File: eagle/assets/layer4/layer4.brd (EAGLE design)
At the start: 102.9 x 102.9 mm, 45 parts, among them Y1 8MHz

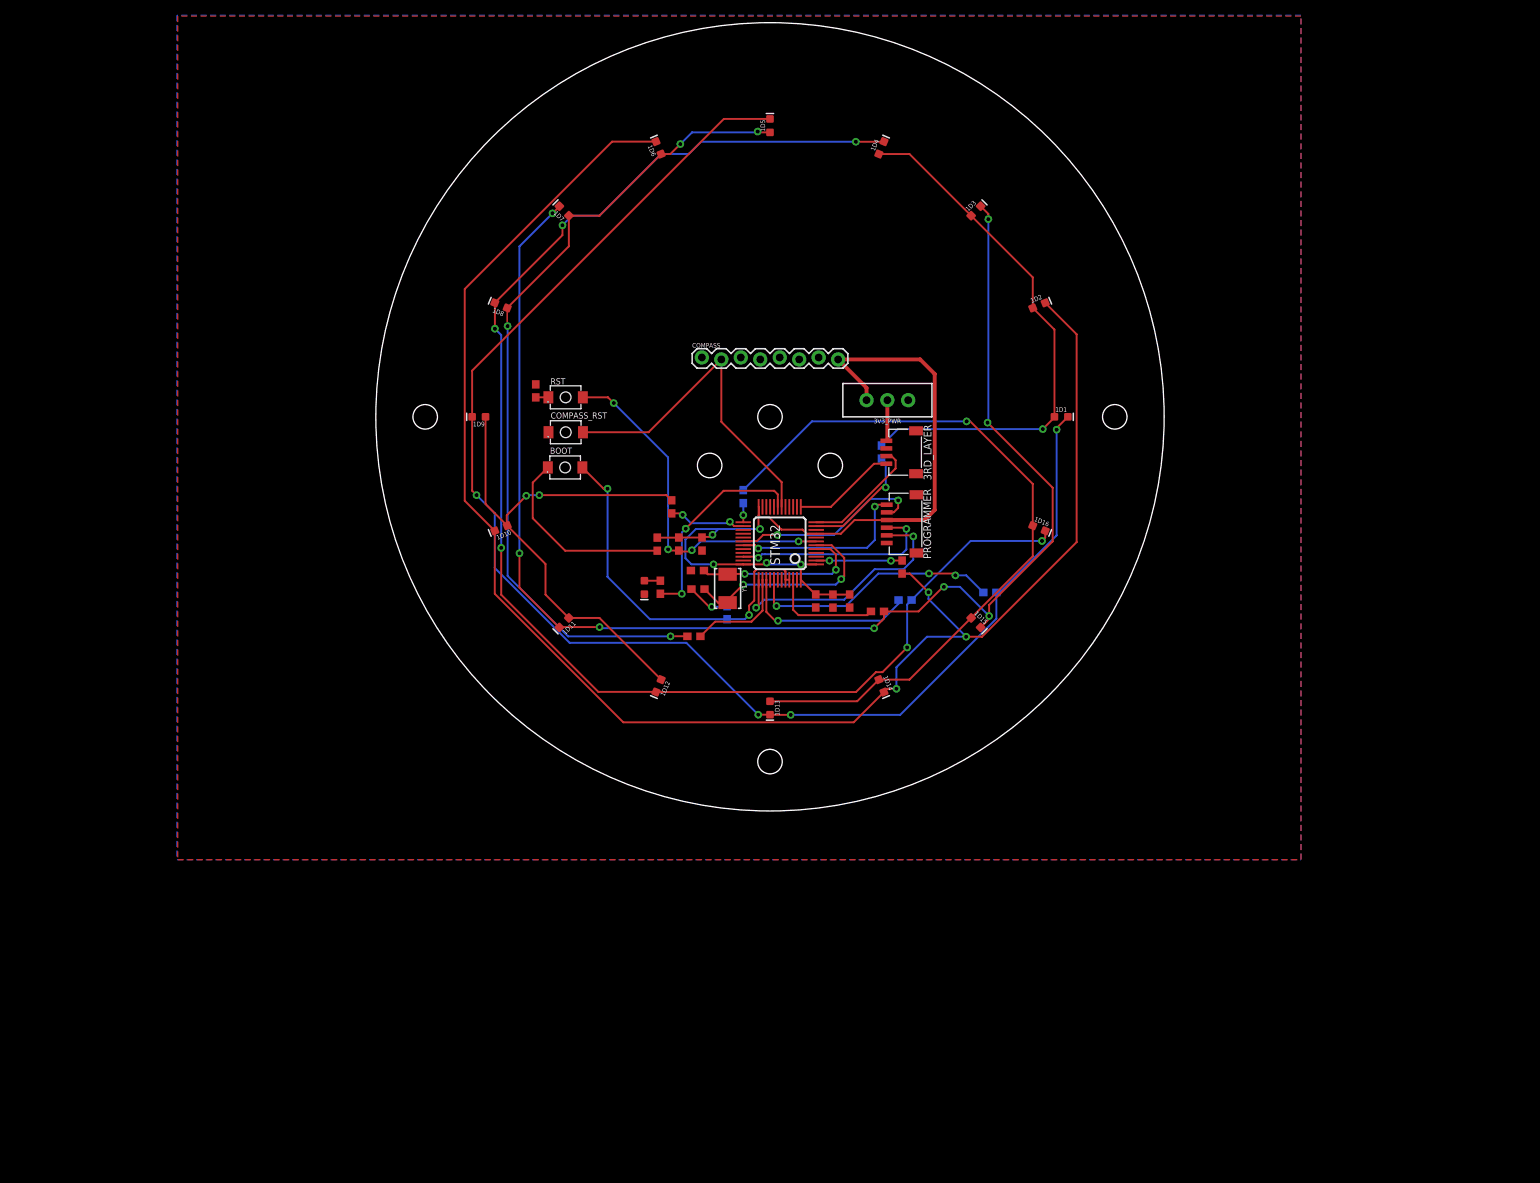
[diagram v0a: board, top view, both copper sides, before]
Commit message: ??
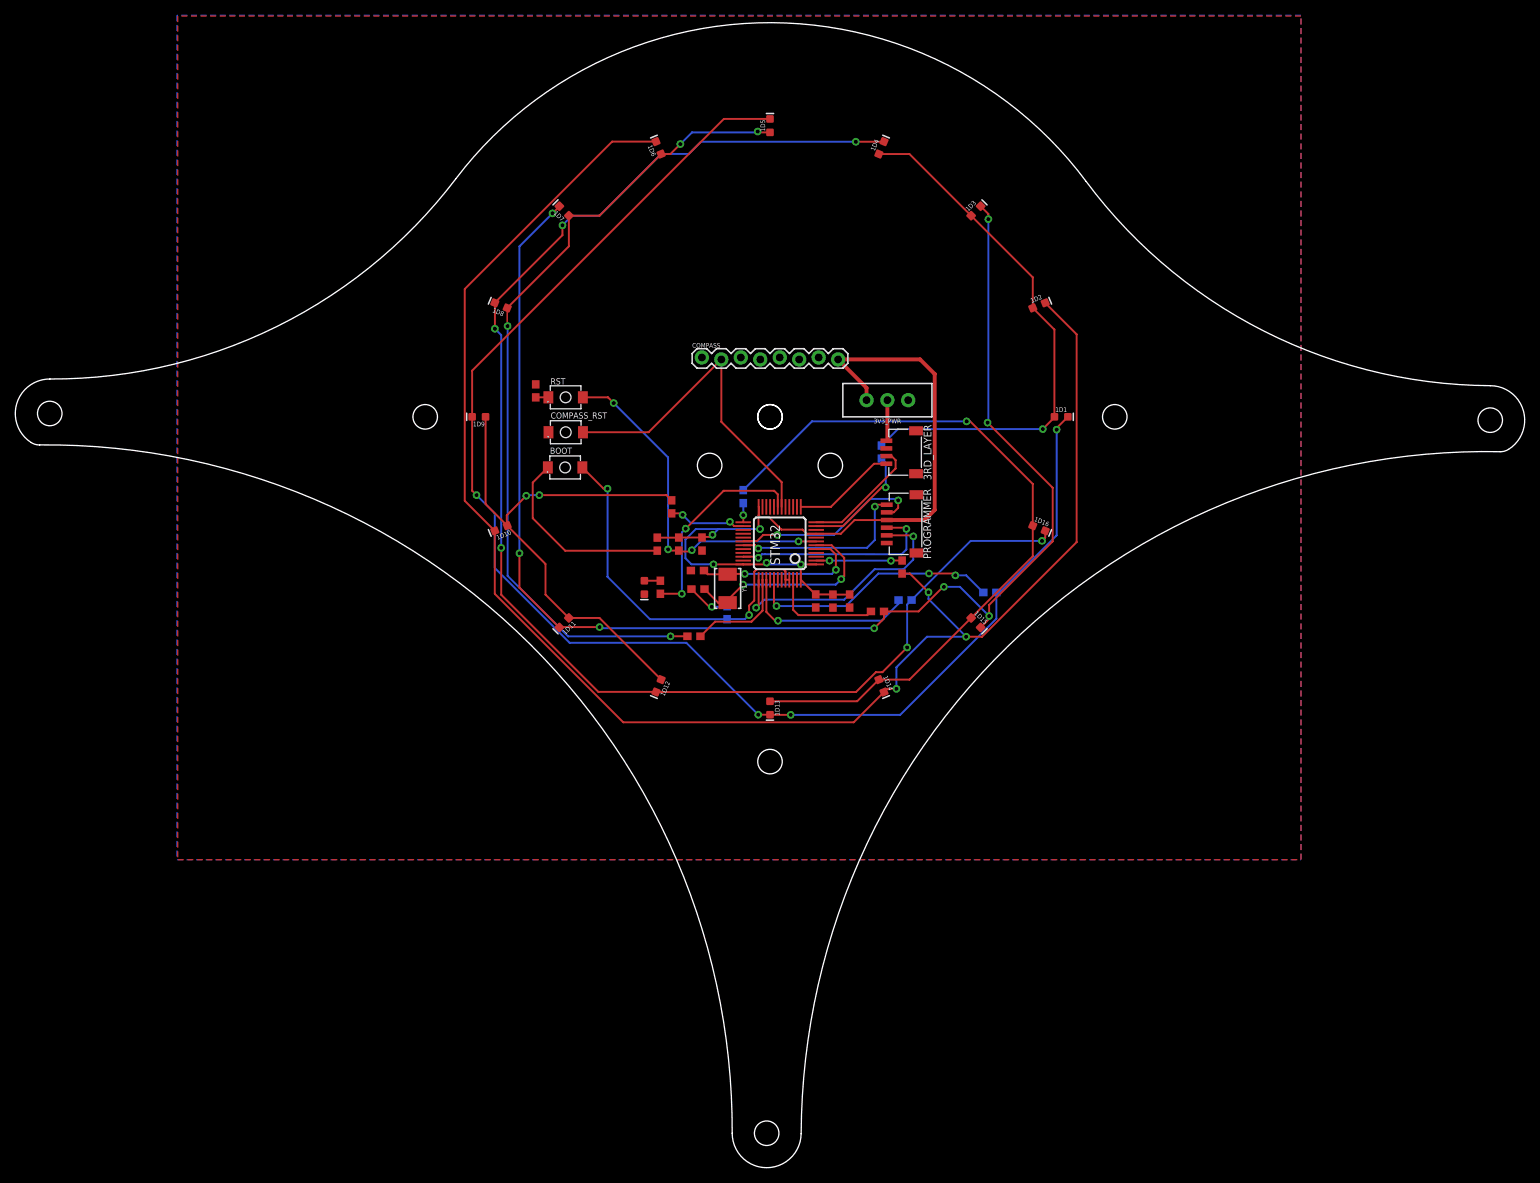
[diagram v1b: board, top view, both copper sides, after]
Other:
- board size 102.9 x 102.9 mm -> 197 x 149.4 mm
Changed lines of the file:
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@@
 <board>
 <plain>
-<circle x="0" y="0" radius="51.441709375" width="0.001" layer="20"/>
 <circle x="0" y="0" radius="1.6" width="0.001" layer="20"/>
 <circle x="0" y="-45" radius="1.6" width="0.001" layer="20"/>
@@
 <circle x="0" y="-45" radius="3.54114375" width="0.1524" layer="39"/>
 <circle x="-45" y="0" radius="3.54114375" width="0.1524" layer="39"/>
+<circle x="93.998990625" y="-0.435540625" radius="1.6" width="0.001" layer="20"/>
+<circle x="0" y="0" radius="1.6" width="0.001" layer="20"/>
+<circle x="-0.43323125" y="-93.499" radius="1.6" width="0.001" layer="20"/>
+<circle x="-93.998990625" y="0.435540625" radius="1.6" width="0.001" layer="20"/>
+<wire x1="-95.326390625" y1="-3.66913125" x2="-96.427240625" y2="-3.35308125" width="0.001" layer="20" curve="-33.28"/>
+<wire x1="-96.427240625" y1="-3.35308125" x2="-93.978140625" y2="4.935490625" width="0.001" layer="20" curve="-147.61"/>
+<wire x1="-93.978140625" y1="4.935490625" x2="-40.97853125" y2="31.09678125" width="0.001" layer="20" curve="53.07"/>
+<wire x1="-40.97853125" y1="31.09678125" x2="41.264940625" y2="30.715709375" width="0.001" layer="20" curve="-106.14"/>
+<wire x1="41.264940625" y1="30.715709375" x2="94.019840625" y2="4.064409375" width="0.001" layer="20" curve="53.07"/>
+<wire x1="94.019840625" y1="4.064409375" x2="96.39201875" y2="-4.2465" width="0.001" layer="20" curve="-147.61"/>
+<wire x1="96.39201875" y1="-4.2465" x2="95.2883" y2="-4.552340625" width="0.001" layer="20" curve="-33.28"/>
+<wire x1="95.2883" y1="-4.552340625" x2="4.06651875" y2="-93.54716875" width="0.001" layer="20" curve="90.88"/>
+<wire x1="4.06651875" y1="-93.54716875" x2="-4.93321875" y2="-93.50546875" width="0.001" layer="20" curve="-179.3"/>
+<wire x1="-4.93321875" y1="-93.50546875" x2="-95.326390625" y2="-3.66913125" width="0.001" layer="20" curve="90.88"/>
+<circle x="93.974" y="-0.35" radius="3.54114375" width="0.1524" layer="39"/>
+<circle x="-94.026" y="0.45" radius="3.54114375" width="0.1524" layer="39"/>
 </plain>
 <attributes>
